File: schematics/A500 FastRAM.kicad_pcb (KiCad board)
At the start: 2 copper layers, 87.6 x 87.6 mm, 31 parts, among them J1 Microsemi_FlashPro-JTAG-10, U1 68000 Boardside, U10 TPS7333QP, U2 68000 Socket, U3 ATF1502ASV-15JU44, U4 74157, U5 74157, U6 IS41LV16100D, U7 IS41LV16100D, U8 IS41LV16100D, U9 IS41LV16100D

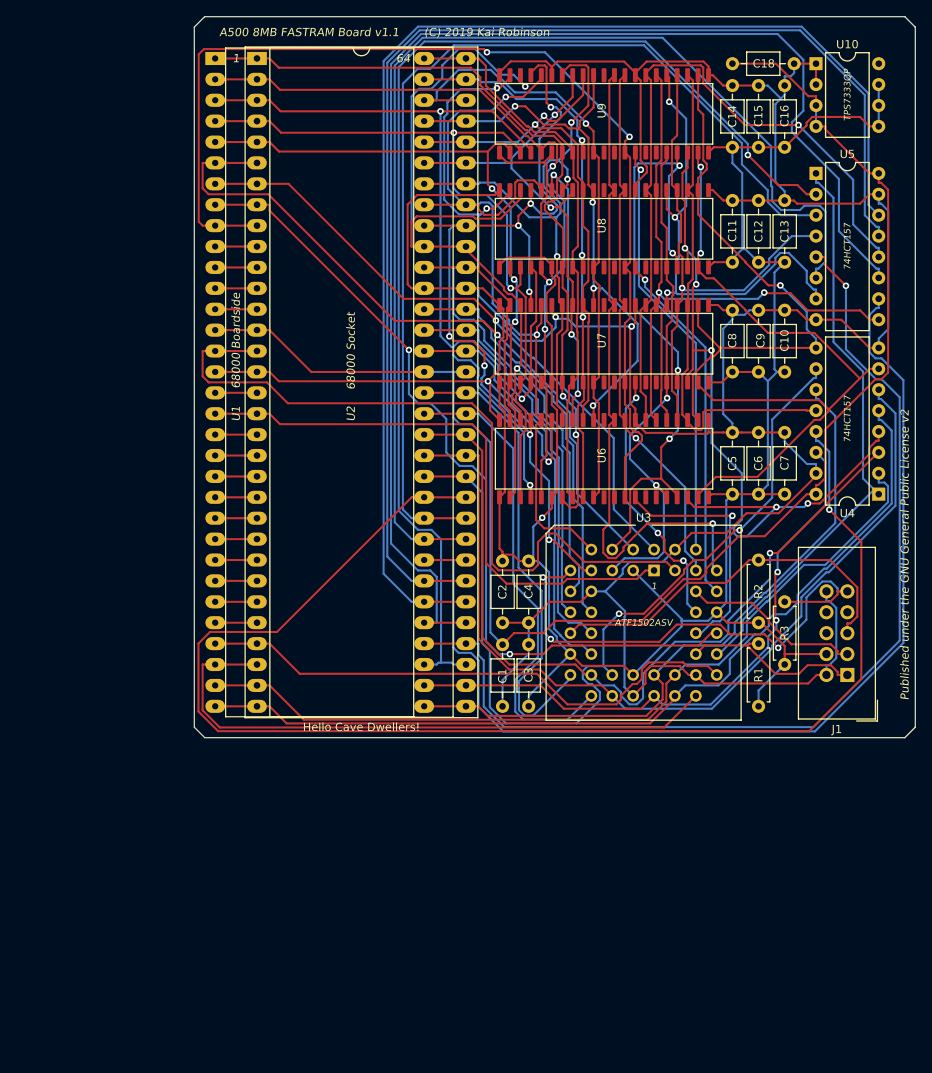
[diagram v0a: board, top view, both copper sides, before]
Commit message: New & Improved ?
Whee! Complete revamp including 14Mhz accelerator!
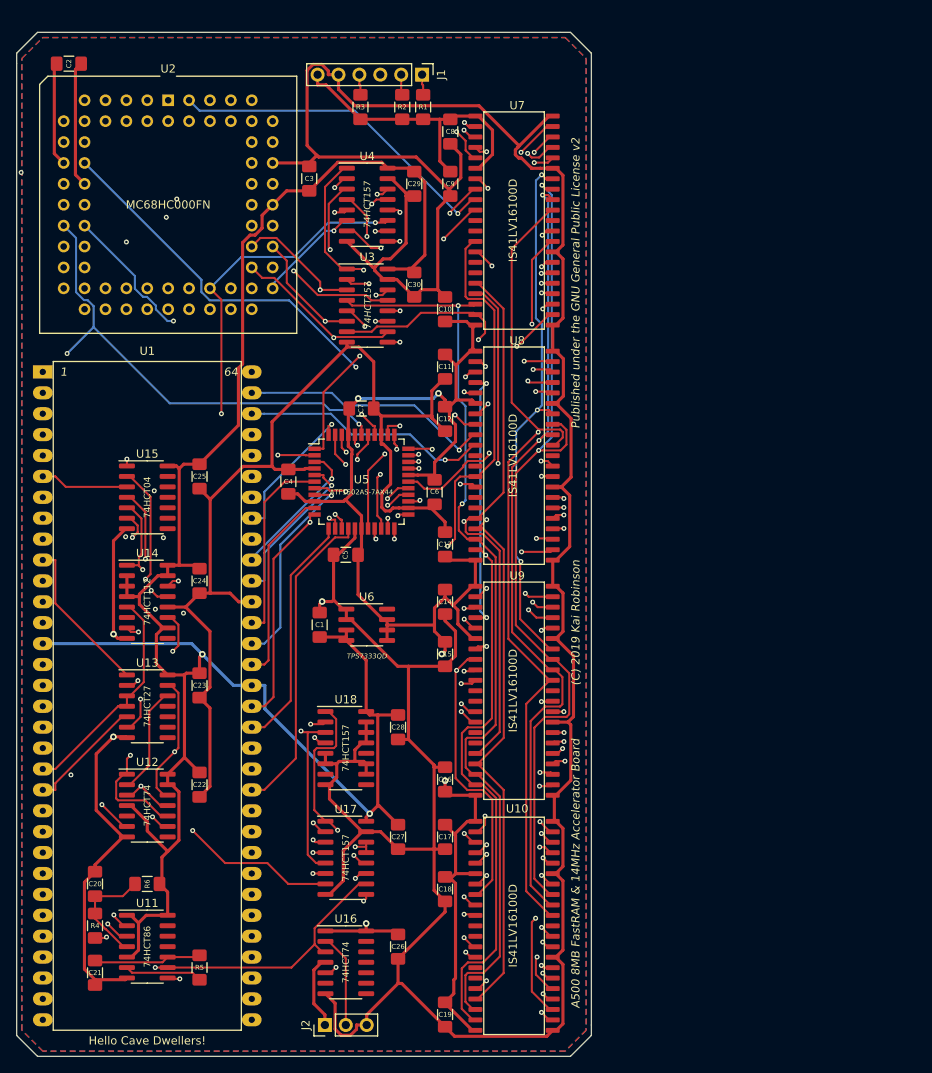
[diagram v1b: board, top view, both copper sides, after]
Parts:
- added C17: 0.1uF, Capacitor_SMD:C_1206_3216Metric_Pad1.42x1.75mm_HandSolder, F.Cu at (148.6, 130.2)
- added C19: 0.1uF, Capacitor_SMD:C_1206_3216Metric_Pad1.42x1.75mm_HandSolder, F.Cu at (148.6, 151.8)
- added C20: 22pf, Capacitor_SMD:C_1206_3216Metric_Pad1.42x1.75mm_HandSolder, F.Cu at (106.0, 135.9)
- added C21: 22pf, Capacitor_SMD:C_1206_3216Metric_Pad1.42x1.75mm_HandSolder, F.Cu at (106.0, 146.7)
- added C22: 0.1uF, Capacitor_SMD:C_1206_3216Metric_Pad1.42x1.75mm_HandSolder, F.Cu at (118.7, 123.8)
- added C23: 0.1uF, Capacitor_SMD:C_1206_3216Metric_Pad1.42x1.75mm_HandSolder, F.Cu at (118.7, 111.8)
- added C24: 0.1uF, Capacitor_SMD:C_1206_3216Metric_Pad1.42x1.75mm_HandSolder, F.Cu at (118.7, 99.1)
- added C25: 0.1uF, Capacitor_SMD:C_1206_3216Metric_Pad1.42x1.75mm_HandSolder, F.Cu at (118.7, 86.4)
- added C26: 0.1uF, Capacitor_SMD:C_1206_3216Metric_Pad1.42x1.75mm_HandSolder, F.Cu at (142.9, 143.5)
- added C27: 0.1uF, Capacitor_SMD:C_1206_3216Metric_Pad1.42x1.75mm_HandSolder, F.Cu at (142.9, 130.2)
- added C28: 0.1uF, Capacitor_SMD:C_1206_3216Metric_Pad1.42x1.75mm_HandSolder, F.Cu at (142.9, 116.8)
- added C29: 0.1uF, Capacitor_SMD:C_1206_3216Metric_Pad1.42x1.75mm_HandSolder, F.Cu at (144.8, 50.8)
- added C30: 0.1uF, Capacitor_SMD:C_1206_3216Metric_Pad1.42x1.75mm_HandSolder, F.Cu at (144.8, 63.1)
- added J2: Speed Selector, Connector_PinHeader_2.54mm:PinHeader_1x03_P2.54mm_Vertical, F.Cu at (134.0, 153.0)
- added R4: 560, Resistor_SMD:R_1206_3216Metric_Pad1.42x1.75mm_HandSolder, F.Cu at (106.0, 141.0)
- added R5: 560, Resistor_SMD:R_1206_3216Metric_Pad1.42x1.75mm_HandSolder, F.Cu at (118.7, 146.1)
- added R6: 10k, Resistor_SMD:R_1206_3216Metric_Pad1.42x1.75mm_HandSolder, F.Cu at (112.4, 135.9)
- added U11: 74HC86, Package_SO:SOIC-14_3.9x8.7mm_P1.27mm, F.Cu at (112.4, 143.5)
- added U12: 74HC74, Package_SO:SOIC-14_3.9x8.7mm_P1.27mm, F.Cu at (112.4, 126.4)
- added U13: 74LS27, Package_SO:SOIC-14_3.9x8.7mm_P1.27mm, F.Cu at (112.4, 114.3)
- added U14: 74LS112, Package_SO:SOIC-16_3.9x9.9mm_P1.27mm, F.Cu at (112.4, 101.6)
- added U15: 74HC04, Package_SO:SOIC-14_3.9x8.7mm_P1.27mm, F.Cu at (112.4, 88.9)
- added U16: 74HC74, Package_SO:SOIC-14_3.9x8.7mm_P1.27mm, F.Cu at (136.5, 145.4)
- added U17: 74LS157, Package_SO:SOIC-16_3.9x9.9mm_P1.27mm, F.Cu at (136.5, 132.7)
- added U18: 74LS157, Package_SO:SOIC-16_3.9x9.9mm_P1.27mm, F.Cu at (136.5, 119.4)
- C1, C10, C11, C12, C13, C14, C15, C16, C18, C2, C3, C4, C5, C6, C7, C8, C9: footprint Capacitor_THT:C_Axial_L3.8mm_D2.6mm_P7.50mm_Horizontal -> Capacitor_SMD:C_1206_3216Metric_Pad1.42x1.75mm_HandSolder
- J1: value Microsemi_FlashPro-JTAG-10 -> Conn_01x06_Male; footprint Connector_IDC:IDC-Header_2x05_P2.54mm_Vertical -> Connector_PinHeader_2.54mm:PinHeader_1x06_P2.54mm_Vertical
- R1, R2, R3: footprint Resistor_THT:R_Axial_DIN0207_L6.3mm_D2.5mm_P7.62mm_Horizontal -> Resistor_SMD:R_1206_3216Metric_Pad1.42x1.75mm_HandSolder
- U10: value TPS7333QP -> IS41LV16100D; footprint Package_DIP:DIP-8_W7.62mm -> Package_SO_J-Lead:SOJ-42
- U2: value 68000 Socket -> MC68000FN; footprint Package_DIP:DIP-64_W25.4mm_Socket_LongPads -> Package_LCC:PLCC-68_THT-Socket
- U3: value ATF1502ASV-15JU44 -> 74157; footprint Package_LCC:PLCC-44_THT-Socket -> Package_SO:SOIC-16_3.9x9.9mm_P1.27mm
- U4: footprint Package_DIP:DIP-16_W7.62mm -> Package_SO:SOIC-16_3.9x9.9mm_P1.27mm
- U5: value 74157 -> ATF1502AS-7AX44; footprint Package_DIP:DIP-16_W7.62mm -> Package_QFP:TQFP-44_10x10mm_P0.8mm
- U6: value IS41LV16100D -> TPS7333QD; footprint Package_SO_J-Lead:SOJ-42 -> Package_SO:SOIC-8_3.9x4.9mm_P1.27mm
- moved U10 109.5 mm to (157.4, 139.4)
- moved C18 106.2 mm to (148.6, 136.5), turned to 270 degrees
- moved J1 89.4 mm to (145.8, 37.5), turned to 270 degrees
- moved C16 87.2 mm to (148.6, 123.2)
- moved C2 86.0 mm to (102.9, 36.2), turned to 180 degrees
- moved R3 85.1 mm to (138.3, 41.5)
- moved R1 83.5 mm to (145.9, 41.5)
- moved R2 76.2 mm to (143.4, 41.5)
- moved C15 72.4 mm to (148.6, 108.0), turned to 270 degrees
- moved U4 71.4 mm to (139.1, 53.3), turned to 0 degrees
- moved U9 69.5 mm to (157.4, 110.9), turned to 0 degrees
- moved C3 69.5 mm to (132.1, 50.2), turned to 270 degrees
- moved U5 66.8 mm to (138.4, 87.0)
- moved C14 65.4 mm to (148.6, 101.6), turned to 270 degrees
- moved C13 53.7 mm to (148.6, 94.6)
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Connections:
- C18 pad 1: VCC -> /VCC33
- C2 pad 2: /VCC33 -> VCC
- C3 pad 1: /VCC33 -> GND
- C3 pad 2: GND -> VCC
- C6 pad 1: /VCC33 -> GND
- C6 pad 2: GND -> /VCC33
- C7 pad 1: /VCC33 -> GND
- C7 pad 2: GND -> /VCC33
- J1 pad 1: /TCK -> /TMS
- J1 pad 2: GND -> /TDI
- J1 pad 4: /VCC33 -> /TCK
- J1 pad 5: /TMS -> GND
- J1 pad 6: Net-(J1-Pad6) -> /VCC33
- R1 pad 2: /TCK -> /TMS
- R2 pad 2: /TMS -> /TDI
- R3 pad 2: /TDI -> /TCK
- U10 pad 1: GND -> /VCC33
- U10 pad 2: GND -> /CPU_D0
- U10 pad 3: VCC -> /CPU_D1
- U10 pad 4: VCC -> /CPU_D2
- U10 pad 5: /VCC33 -> /CPU_D3
- U10 pad 7: /VCC33 -> /CPU_D4
- U10 pad 8: Net-(U10-Pad8) -> /CPU_D5
- U2 pad 10: /CPU_DTACK -> /CPU_DTACK14
- U2 pad 15: /CPU_CLK -> /CPU_CLK14
- U2 pad 17: /CPU_HALT -> GND
- U2 pad 18: /CPU_RESET -> Net-(U2-Pad18)
- U2 pad 19: /CPU_VMA -> /CPU_HALT
- U2 pad 20: /CPU_E -> /CPU_RESET
- U2 pad 21: /CPU_VPA -> /CPU_VMA14
- U2 pad 22: /CPU_BERR -> /CPU_E14
- U2 pad 23: /CPU_IPL2 -> /CPU_VPA14
- U2 pad 24: /CPU_IPL1 -> /CPU_BERR
- U2 pad 25: /CPU_IPL0 -> /CPU_IPL2
- U2 pad 26: /CPU_FC2 -> /CPU_IPL1
- U2 pad 27: /CPU_FC1 -> /CPU_IPL0
- U2 pad 28: /CPU_FC0 -> /CPU_FC2
- U2 pad 29: /CPU_A1 -> /CPU_FC1
- U2 pad 30: /CPU_A2 -> /CPU_FC0
- U2 pad 31: /CPU_A3 -> Net-(U2-Pad31)
- U2 pad 32: /CPU_A4 -> /CPU_A1
- U2 pad 33: /CPU_A5 -> /CPU_A2
- U2 pad 34: /CPU_A6 -> /CPU_A3
- U2 pad 35: /CPU_A7 -> /CPU_A4
- U2 pad 36: /CPU_A8 -> /CPU_A5
- U2 pad 37: /CPU_A9 -> /CPU_A6
- U2 pad 38: /CPU_A10 -> /CPU_A7
- U2 pad 39: /CPU_A11 -> /CPU_A8
- U2 pad 40: /CPU_A12 -> /CPU_A9
- U2 pad 41: /CPU_A13 -> /CPU_A10
- U2 pad 42: /CPU_A14 -> /CPU_A11
- U2 pad 43: /CPU_A15 -> /CPU_A12
- U2 pad 44: /CPU_A16 -> /CPU_A13
- U2 pad 45: /CPU_A17 -> /CPU_A14
- U2 pad 46: /CPU_A18 -> /CPU_A15
- U2 pad 47: /CPU_A19 -> /CPU_A16
- U2 pad 48: /CPU_A20 -> /CPU_A17
- U2 pad 49: VCC -> /CPU_A18
- U2 pad 50: /CPU_A21 -> /CPU_A19
- U2 pad 51: /CPU_A22 -> /CPU_A20
- U2 pad 52: /CPU_A23 -> VCC
- U2 pad 53: GND -> /CPU_A21
- U2 pad 54: /CPU_D15 -> /CPU_A22
- U2 pad 55: /CPU_D14 -> /CPU_A23
- U2 pad 56: /CPU_D13 -> GND
- U2 pad 57: /CPU_D12 -> GND
- U2 pad 58: /CPU_D11 -> /CPU_D15
- U2 pad 59: /CPU_D10 -> /CPU_D14
- U2 pad 6: /CPU_AS -> /CPU_AS14
- U2 pad 60: /CPU_D9 -> /CPU_D13
- U2 pad 61: /CPU_D8 -> /CPU_D12
- U2 pad 62: /CPU_D7 -> /CPU_D11
- U2 pad 63: /CPU_D6 -> /CPU_D10
- U2 pad 64: /CPU_D5 -> /CPU_D9
- U3 pad 1: /CPU_RESET -> /MUX_SWITCH
- U3 pad 10: GND -> /CPU_A16
- U3 pad 11: /CPU_D15 -> /CPU_A5
- U3 pad 12: /CPU_A23 -> /DRAM_A5
- U3 pad 13: /TMS -> /CPU_A15
- U3 pad 14: /CPU_A22 -> /CPU_A6
- U3 pad 15: /VCC33 -> GND
- U3 pad 16: /CPU_A21 -> VCC
- U3 pad 2: /CPU_AS -> /CPU_A3
- U3 pad 3: /VCC33 -> /CPU_A18
- U3 pad 4: /DRAM_A1 -> /DRAM_A2
- U3 pad 5: /DRAM_A0 -> /CPU_A4
- U3 pad 6: /CPU_D12 -> /CPU_A17
- U3 pad 7: /TDI -> /DRAM_A3
- U3 pad 8: /CPU_D13 -> GND
- U3 pad 9: /CPU_D14 -> /DRAM_A4
- U4 pad 10: /CPU_A16 -> /CPU_A12
- U4 pad 11: /CPU_A5 -> /CPU_A9
- U4 pad 12: /DRAM_A5 -> /DRAM_A9
- U4 pad 13: /CPU_A15 -> /CPU_A11
- U4 pad 14: /CPU_A6 -> /CPU_A10
- U4 pad 2: /CPU_A3 -> /CPU_A7
- U4 pad 3: /CPU_A18 -> /CPU_A14
- U4 pad 4: /DRAM_A2 -> /DRAM_A6
- U4 pad 5: /CPU_A4 -> /CPU_A8
- U4 pad 6: /CPU_A17 -> /CPU_A13
- U4 pad 7: /DRAM_A3 -> /DRAM_A7
- U4 pad 9: /DRAM_A4 -> /DRAM_A8
- U5 pad 1: /MUX_SWITCH -> /TDI
- U5 pad 10: /CPU_A12 -> /CPU_A21
- U5 pad 11: /CPU_A9 -> /CPU_A20
- U5 pad 12: /DRAM_A9 -> /CPU_A19
- U5 pad 13: /CPU_A11 -> /CPU_A18
- U5 pad 14: /CPU_A10 -> /CPU_A17
- U5 pad 15: GND -> /CPU_A16
- U5 pad 16: VCC -> GND
- U5 pad 2: /CPU_A7 -> /CPU_D13
- U5 pad 3: /CPU_A14 -> /CPU_D14
- U5 pad 4: /DRAM_A6 -> GND
- U5 pad 5: /CPU_A8 -> /CPU_D15
- U5 pad 6: /CPU_A13 -> /CPU_A23
- U5 pad 7: /DRAM_A7 -> /TMS
- U5 pad 8: GND -> /CPU_A22
- U5 pad 9: /DRAM_A8 -> /VCC33
- U6 pad 1: /VCC33 -> GND
- U6 pad 2: /CPU_D0 -> GND
- U6 pad 3: /CPU_D1 -> VCC
- U6 pad 4: /CPU_D2 -> VCC
- U6 pad 5: /CPU_D3 -> /VCC33
- U6 pad 7: /CPU_D4 -> /VCC33
- U6 pad 8: /CPU_D5 -> Net-(U6-Pad8)
- U7 pad 14: /DRAM_RAS1 -> /DRAM_RAS0
- U8 pad 14: /DRAM_RAS2 -> /DRAM_RAS1
- U9 pad 14: /DRAM_RAS3 -> /DRAM_RAS2
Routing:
- net GND: track 461.4 -> 694.1 mm, vias 5 -> 3
- net VCC: track 184.6 -> 349.5 mm, vias 0 -> 3
- net /CPU_D10: track 62.7 -> 188.9 mm, vias 4 -> 2
- net /CPU_D9: track 65.6 -> 181.5 mm
- net /CPU_AS14: track 0.00 -> 115.3 mm, vias 0 -> 1
- net /CPU_D0: track 83.6 -> 198.9 mm, vias 3 -> 4
- net /CPU_D11: track 73.8 -> 187.0 mm, vias 3 -> 4
- net /CPU_CLK14: track 0.00 -> 110.7 mm, vias 0 -> 2
- net /CPU_D8: track 71.3 -> 181.9 mm, vias 4 -> 1
- net /CPU_E14: track 0.00 -> 101.2 mm, vias 0 -> 2
- net /CPU_D1: track 93.1 -> 194.3 mm, vias 2 -> 4
- net /CPU_VPA14: track 0.00 -> 99.5 mm, vias 0 -> 2
- net /CPU_D5: track 67.9 -> 159.7 mm, vias 0 -> 3
- net /CPU_D6: track 70.5 -> 161.0 mm, vias 3 -> 4
- net /CPU_DTACK14: track 0.00 -> 90.0 mm, vias 0 -> 1
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- added copper zone on B.Cu, net GND
- added copper zone on F.Cu, net GND
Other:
- board size 87.6 x 87.6 mm -> 69.9 x 124.5 mm
- copper layers 2 -> 4
- net class Default: via_dia 0.8 -> 0.6; via_drill 0.4 -> 0.3
- net class Power added: clearance 0.2, trace_width 0.381, via_dia 0.8, via_drill 0.4
- board text added: "74HCT04"
- board text added: "74HCT112"
- board text added: "74HCT27"
- board text added: "74HCT74"
- board text added: "74HCT86"
- board text added: "A500 8MB FastRAM & 14MHz Accelerator Board"
- board text added: "ATF1502AS-7AX44"
- board text added: "IS41LV16100D"
- board text added: "MC68HC000FN"
- board text added: "TPS7333QD"
- board text removed: "1"
- board text removed: "A500 8MB FASTRAM Board v1.1"
- board text removed: "ATF1502ASV"
- board text removed: "TPS7333QP"
